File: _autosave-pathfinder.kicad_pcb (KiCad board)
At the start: 2 copper layers, 90.5 x 114.3 mm, 29 parts, among them SW1 SW_Push, SW2 SW_Push, SW3 SW_Push, SW4 SW_Push, SW5 SW_Push, SW6 SW_Push, SW7 SW_Push, SW8 SW_Push, SW9 SW_Push, U1 XIAO-RP2040-DIP, U2 OLED_0.91_128x32

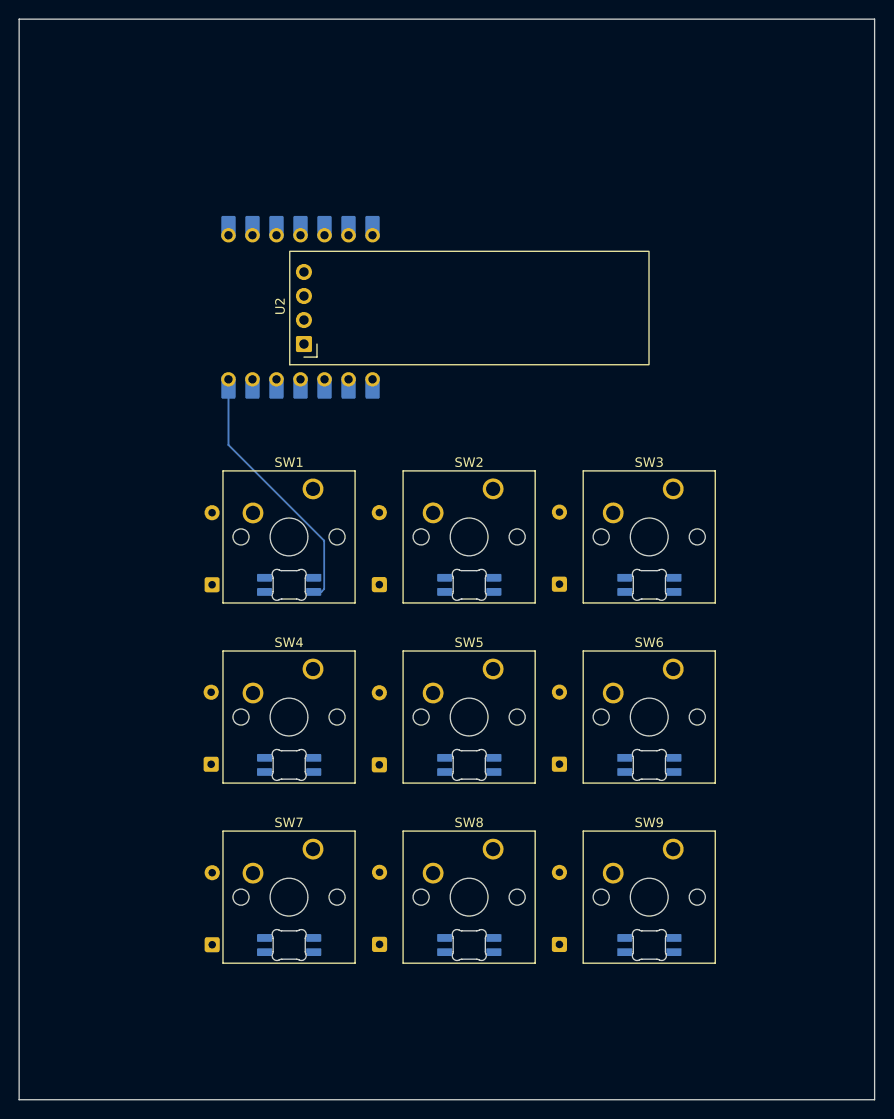
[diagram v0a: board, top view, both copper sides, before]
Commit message: work
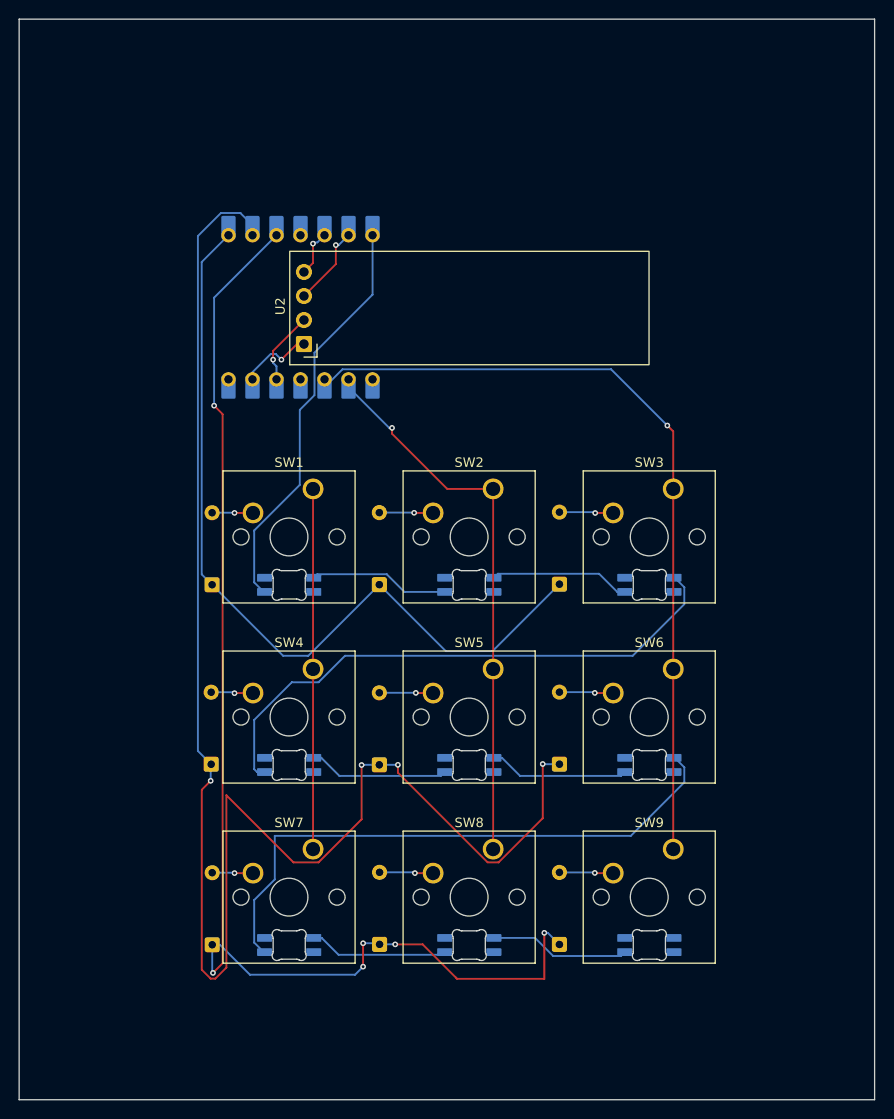
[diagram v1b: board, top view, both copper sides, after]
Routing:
- net ROW2: track 0.00 -> 166.9 mm, vias 0 -> 4
- net ROW3: track 0.00 -> 132.4 mm, vias 0 -> 6
- net ROW1: track 0.00 -> 87.4 mm
- net COL3: track 0.00 -> 84.6 mm, vias 0 -> 1
- net Net-(D15-DOUT): track 0.00 -> 62.5 mm
- net Net-(D12-DOUT): track 0.00 -> 60.3 mm
- net COL2: track 0.00 -> 59.4 mm, vias 0 -> 1
- net DIN1: track 0.00 -> 44.3 mm
- net COL1: track 0.00 -> 38.1 mm
- net VBUS: track 27.6 -> 0.00 mm
- net Net-(D11-DOUT): track 0.00 -> 14.8 mm
- net Net-(D13-DOUT): track 0.00 -> 14.8 mm
- net Net-(D14-DOUT): track 0.00 -> 14.8 mm
- net Net-(D17-DOUT): track 0.00 -> 14.8 mm
- net Net-(D10-DOUT): track 0.00 -> 14.8 mm
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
